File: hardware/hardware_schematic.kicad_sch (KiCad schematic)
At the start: 8 parts, among them SW1 BUTTON, U1 TC1602A-01T, U2 DS18B20

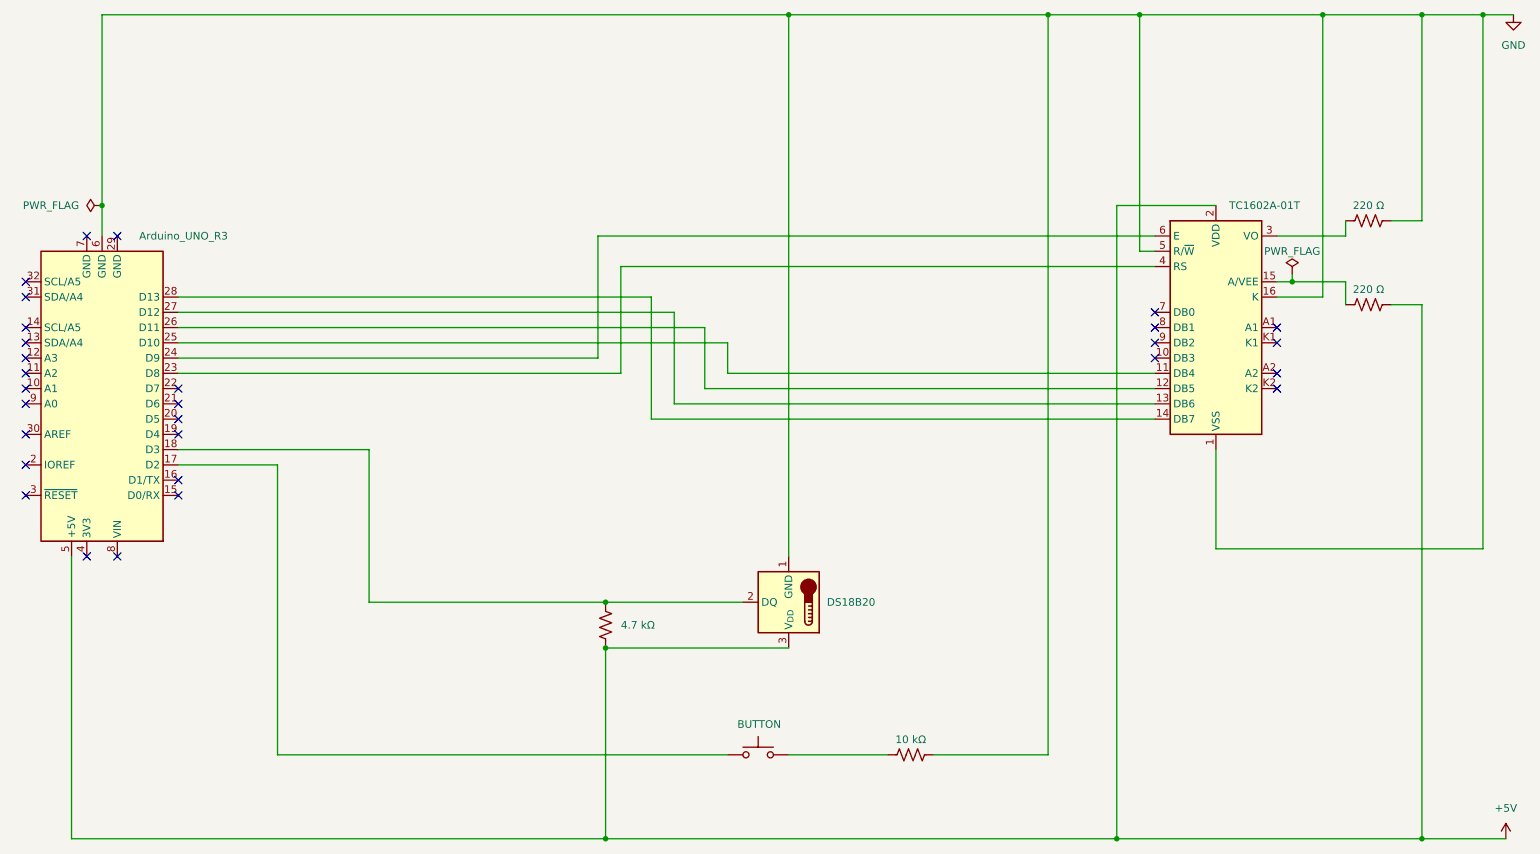
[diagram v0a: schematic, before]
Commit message: hw: correct schematic
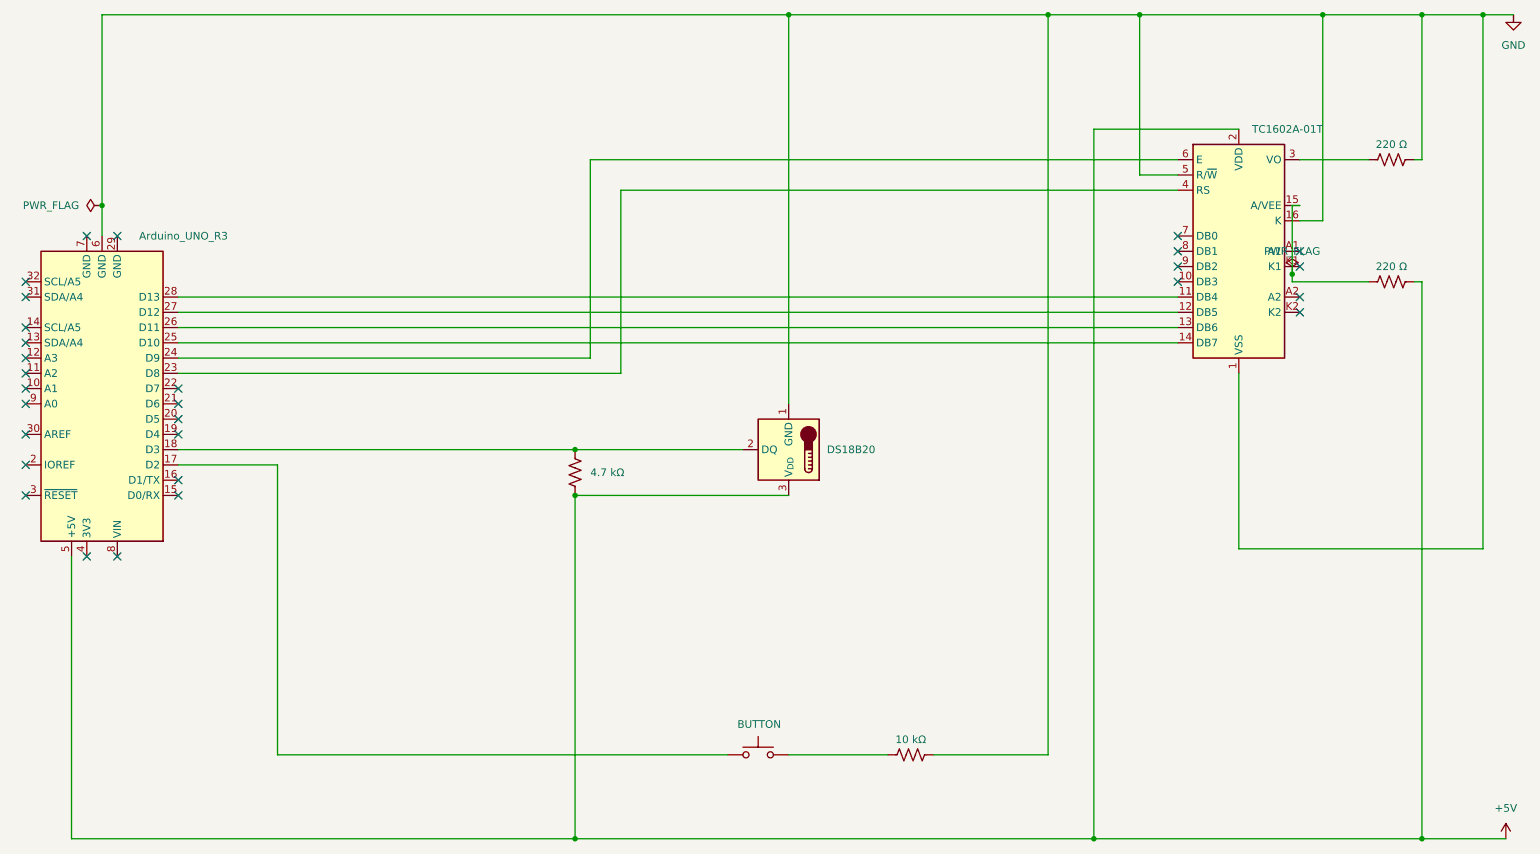
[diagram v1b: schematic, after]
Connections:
- net at U1.11 (DB4): now also A1.28 (D13); no longer A1.25 (D10)
- net at U1.12 (DB5): now also A1.27 (D12); no longer A1.26 (D11)
- net at U1.13 (DB6): now also A1.26 (D11); no longer A1.27 (D12)
- net at U1.14 (DB7): now also A1.25 (D10); no longer A1.28 (D13)
